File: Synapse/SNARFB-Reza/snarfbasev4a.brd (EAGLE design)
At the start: 80 x 49.5 mm, 67 parts, among them J1 AVR_SPI_PRG_6PTH, X1 USBSMD

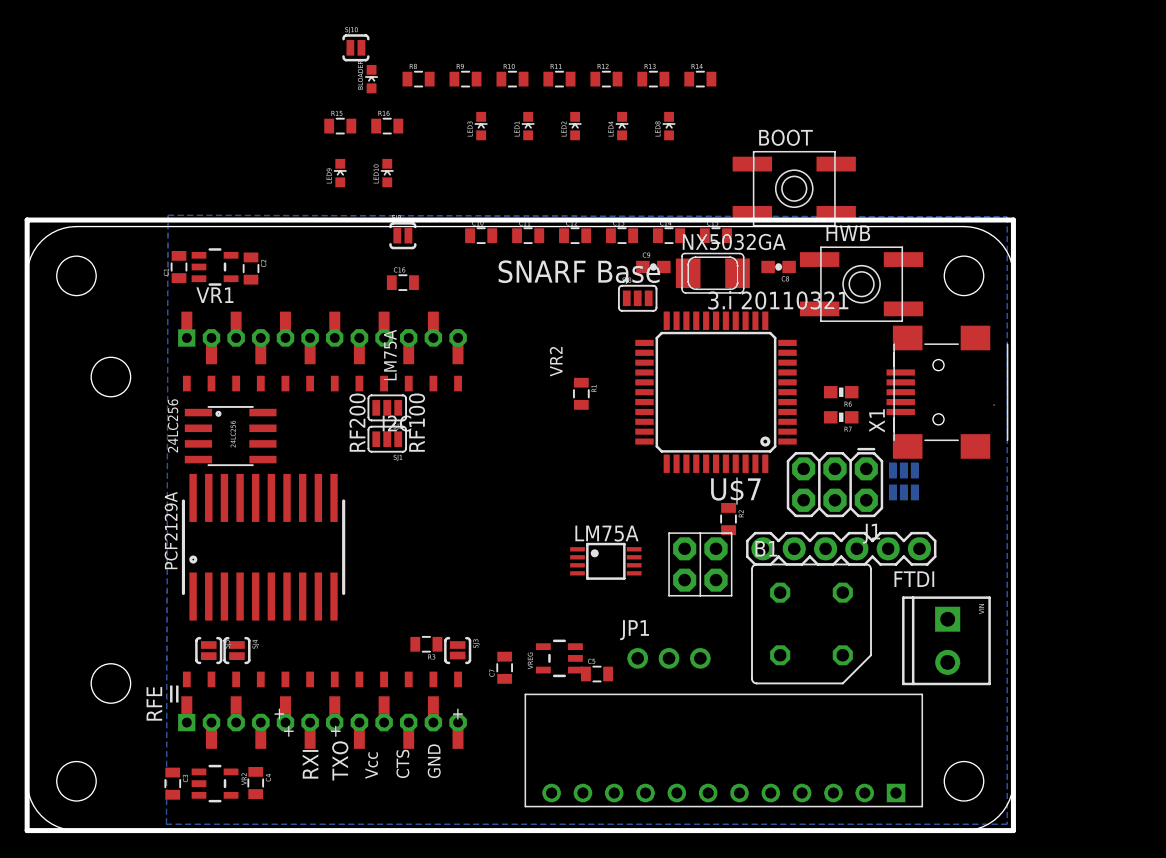
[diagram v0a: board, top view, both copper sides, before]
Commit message: comp sync
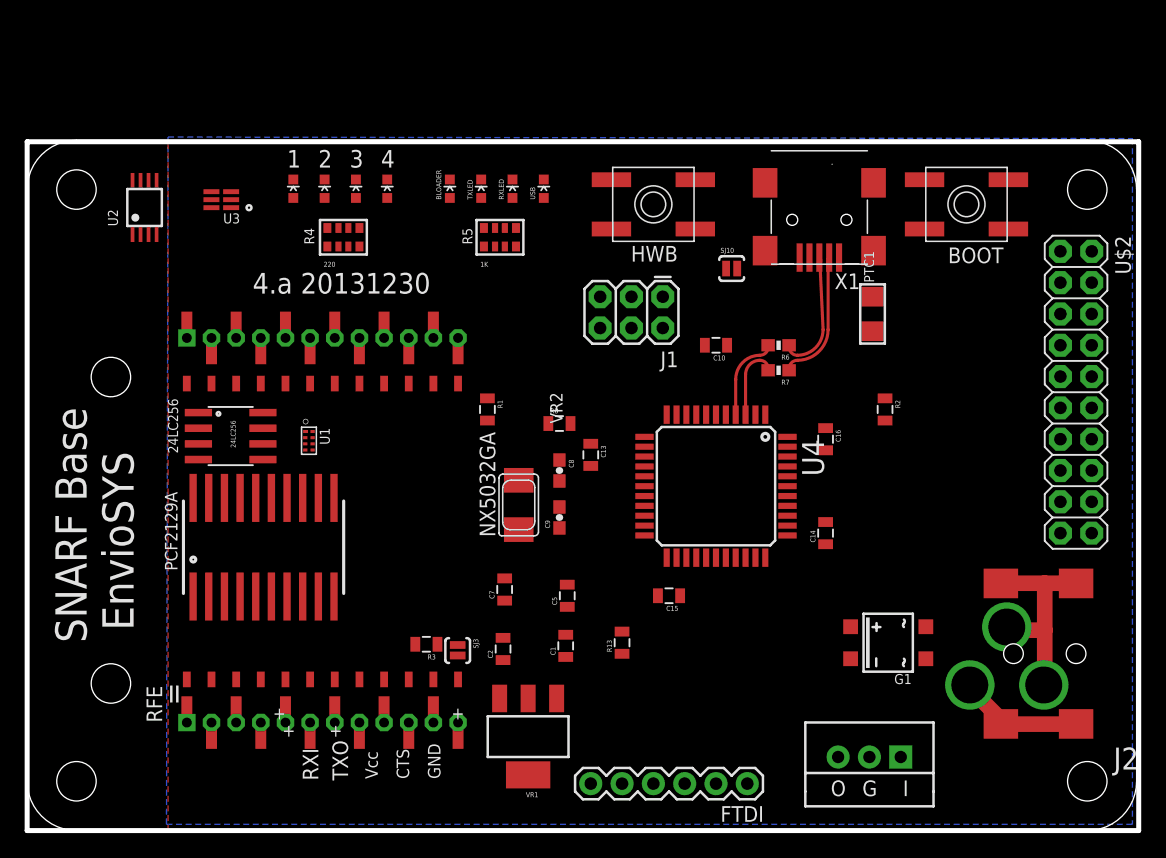
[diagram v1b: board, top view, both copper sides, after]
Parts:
- removed B1: (no value), rectifier:1KAB
- removed C11, C12, C3, C4: 1uF, 0_jc-custom:0805
- removed JP1: (no value), adafruit:1X03-CLEANBIG
- removed LED1: red, 0_jc-custom:LED-0603
- removed LED10: GREEN, 0_jc-custom:LED-0603
- removed LED2: blue, 0_jc-custom:LED-0603
- removed LED3: orange, 0_jc-custom:LED-0603
- removed LED4: green, 0_jc-custom:LED-0603
- removed LED8, LED9: RED, 0_jc-custom:LED-0603
- removed LM75A: LM75AJC-TEST, 0_jc-custom-eagle6:TSSOP8-3MM
- removed PCB1: PCB_DP_RECTANGLE-80X49, dp_pcb:DP8049_V1
- removed R10, R16, R9: 220, SparkFun-Resistors:0805
- removed R11, R12, R14, R15: 1K, SparkFun-Resistors:0805
- removed RXTX: SERIAL_CROSSOVERNORMAL, 0_jc-custom-eagle6:2X02_SXOVER
- removed SJ1, SJ2: (no value), SparkFun:SJ_3
- removed SJ4, SJ5, SJ9: SOLDERJUMPERNO, SparkFun:SJ_2S-NO
- removed SJ6, SJ7: (no value), SparkFun:SJ_3_PASTE1&2
- removed SJ8: (no value), SparkFun:SJ_3_PASTE2&3
- removed U$1: R7XXXDEF, 0_jc-custom-eagle6:1X12_RECOM
- removed U$7: ATMEGA32U4-AU, adafruit:TQFP44
- removed VIN: M023.5MM, SparkFun-Connectors:SCREWTERMINAL-3.5MM-2
- removed VR2, VREG: MCP1802, 0_jc-custom:SOT23-5
- added 1, 2, 3, 4: red, 0_jc-custom:LED-0603
- added G1: (no value), microbuilder:SOIC-4
- added IC1: (no value), 0_jc-custom-eagle6:TO220-MURATA
- added J2: POWER_JACKCOMBO, SparkFun-Connectors:POWER_JACK_COMBO
- added PTC1: (no value), microbuilder:1206
- added R4: 220, microbuilder:RESPACK_4X0603
- added R5: 1K, microbuilder:RESPACK_4X0603
- added RXLED, TXLED: yellow, 0_jc-custom:LED-0603
- added U$2: M10X2, SparkFun-Connectors:2X10
- added U$3: (no value), dp_pcb:DP9056_V1
- added U1: (no value), microbuilder:SOT833-1
- added U2: lm75adp, microbuilder:TSSOP8
- added U3: TSL2561_DFN, microbuilder:TSL2561_FN
- added U4: ATMEGA32U4-AU, adafruit:TQFP44
- added USB: GREEN, 0_jc-custom:LED-0603
- R3: value (none) -> 10k
- R8: value 220 -> 10K
- VR1: value MCP1802 -> MCP1826S; device 0_jc-custom:SOT23-5 -> SparkFun-PowerIC:SOT223
- moved VR1 45.8 mm to (40.6, 7.62), turned to 180 degrees
- moved R13 45.8 mm to (48.3, 15.2), turned to 90 degrees
- moved C1 43.9 mm to (43.7, 15.0)
- moved C2 37.0 mm to (38.6, 14.7), turned to 90 degrees
- moved C16 36.6 mm to (64.8, 31.8), turned to 270 degrees
- moved SJ10 35.4 mm to (57.1, 45.6)
- moved R8 30.2 mm to (43.2, 33.0)
- moved C15 29.5 mm to (52.1, 19.1), turned to 180 degrees
- moved C14 27.3 mm to (64.8, 24.1), turned to 90 degrees
- moved NX5032GA 24.5 mm to (39.9, 26.4), turned to 90 degrees
- moved C8 24.3 mm to (43.2, 29.2), turned to 270 degrees
- moved FTDI 23.6 mm to (58.4, 3.81)
- moved C9 21.7 mm to (43.2, 25.4), turned to 90 degrees
- moved J1 21.6 mm to (51.6, 43.3)
- moved C10 21.0 mm to (55.9, 39.4), turned to 180 degrees
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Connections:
- net UDM renamed UDM_N
- net UDP renamed UDM_P
- removed net 12VUNREG: B1.+, U$1.P$2, U$1.P$3, U$1.P$4
- removed net 24VAC1: B1.AC2, VIN.1
- removed net 24VAC2: B1.AC1, VIN.2
- removed net FTDI_GND: FTDI.6, SJ7.2
- removed net FTDI_VCC: FTDI.4, SJ6.2
- removed net GPIO10: RFE.12, RFE.P12, RFE.P212, SJ3.2
- removed net GPIO17: RFE.19, RFE.P19, RFE.P219, SJ2.3
- removed net GPIO18: RFE.20, RFE.P20, RFE.P220, SJ1.3
- removed net GPIO7: RFE.9, RFE.P209, RFE.P9, RXTX.4
- removed net GPIO8: RFE.10, RFE.P10, RFE.P210, RXTX.1
- removed net GPIO9: FTDI.5, RFE.11, RFE.P11, RFE.P211
- removed net MVOUT: C12.1, R11.2, SJ9.1, VREG.5
- removed net N$13: LED4.A, R16.2
- removed net PB4-GRN-L4: R16.1, U$7.28
- removed net PB5-ORANGE-L3: R10.1, U$7.29
- removed net PB6-BLUE-L2: R9.1, U$7.30
- removed net PB7-RED-L1: R8.1, U$7.12
- removed net PC6-LED8: LED8.A, U$7.31
- removed net PC7-LED9: LED9.A, U$7.32
- removed net PD4: U$7.25
- removed net PD5: U$7.22
- removed net PD6: U$7.26
- removed net PD7: U$7.27
- removed net PE6-LED7-BOOTLOADER: BLOADER.A, U$7.1
- removed net PF0-2: U$7.41
- removed net PF1-3: U$7.40
- removed net PF4-4: U$7.39
- removed net PF5-5: U$7.38
- removed net PF6-6: U$7.37
- removed net PF7-7: U$7.36
- removed net SCL: 24LC256.6, LM75A.2, PCF2129A.P$1, R1.1, SJ1.2, SJ4.1, U$7.18
- removed net SDA: 24LC256.5, LM75A.1, PCF2129A.P$4, R2.1, SJ2.2, SJ5.1, U$7.19
- removed net SD_CS: U$7.8
- removed net UD+: R6.2, U$7.4
- removed net UD-: R7.2, U$7.3
- removed net VCC3A: C4.1, VR2.5
- new net ARXLED: RXLED.C, U4.8
- new net ATXLED: TXLED.C, U4.22
- new net LINT: U3.INT
- new net N$12: 4.A, R4.5
- new net N$3: G1.~1, J2.POWER
- new net PB4-L4-D8: R4.4, U4.28
- new net PB5-L3-D9: R4.3, U4.29
- new net PB6-L2-D10: R4.2, U4.30
- new net PB7-L1-D11: R4.1, U4.12
- new net PC6-D5: U$2.16, U4.31
- new net PC7-D13-LED9BLOAD: BLOADER.C, U4.32
- new net PD4-D4-GPIO10: RFE.12, RFE.P12, RFE.P212, U4.25
- new net PD6-D12-I2COE: U1.6, U4.26
- new net PD7-D6: U$2.18, U4.27
- new net PE6-D7-GPIO9: FTDI.5, RFE.11, RFE.P11, RFE.P211, U4.1
- new net PF0-A5: U$2.4, U4.41
- new net PF1-A4: U$2.6, U4.40
- new net PF4-A3: U$2.8, U4.39
- new net PF5-A2: U$2.10, U4.38
- new net PF6-A1: U$2.12, U4.37
- new net PF7-A0: U$2.14, U4.36
- new net SCL3: 24LC256.6, PCF2129A.P$1, R1.1, RFE.20, RFE.P20, RFE.P220, U1.4, U2.2, U3.CLK
- new net SCL5: U1.1, U4.18
- new net SDA3: 24LC256.5, PCF2129A.P$4, R2.1, RFE.19, RFE.P19, RFE.P219, U1.5, U2.1, U3.DATA
- new net SDA5: U1.8, U4.19
- new net UD_N: R7.2, U4.3
- new net UD_P: R6.2, U4.4
- new net VBUSRAW: PTC1.2, X1.VBUS
- net AREF-7: now also U4.42; no longer U$7.42
- net GND: now also 1.C, 2.C, 3.C, 4.C, FTDI.6, G1.-, IC1.GND, U$2.19, U$2.20, U1.2, U2.4, U2.5, U2.6, U2.7, U3.ADR, U3.VSS, U4.15, U4.23, U4.35, U4.43, U4.5, USB.C, VR1.4; no longer B1.-, C11.2, C12.2, C3.2, C4.2, JP1.2, LED1.C, LED10.C, LED2.C, LED3.C, LED4.C, LM75A.4, LM75A.5, LM75A.6, LM75A.7, R12.2, R14.2, R15.2, SJ6.3, SJ7.1, U$1.P$5, U$1.P$6, U$1.P$7, U$1.P$8, U$7.15, U$7.23, U$7.35, U$7.43, U$7.5, VR2.2, VREG.2, X1.GND
- net GPIO0: now also SJ3.2; no longer SJ5.2
- net GPIO1: now also U2.3; no longer SJ4.2
- net GPIO11: no longer SJ1.1
- net GPIO12: no longer SJ2.1
- net GPIO13: now also U$2.15
- net GPIO14: now also U$2.13
- net GPIO15: now also U$2.9
- net GPIO16: now also U$2.11
- net GPIO2: now also U$2.3
- net GPIO5: now also U$2.5; no longer VR2.3
- net GPIO6: now also U$2.7
- net HWB: now also U4.33; no longer U$7.33
- net MISO: now also U4.11; no longer U$7.11
- net MOSI: now also U4.10; no longer U$7.10
- net N$1: now also 1.A, R4.8; no longer LED2.A, R9.2
- net N$10: now also R5.5, USB.A; no longer BLOADER.C, R12.1
- net N$11: now also X1.GND; no longer LM75A.3
- net N$2: now also 2.A, R4.7; no longer LED3.A, R10.2
- net N$4: now also U4.6; no longer U$7.6
- net N$5: now also BLOADER.A, R5.8; no longer LED9.C, R15.1
- net N$6: now also 3.A, R4.6; no longer LED1.A, R8.2
- net N$7: now also G1.~2, J2.GND, J2.GND@1; no longer FTDI.1
- net N$8: now also R5.7, TXLED.A; no longer LED10.A, R11.1
- net N$9: now also R5.6, RXLED.A; no longer LED8.C, R14.1
- net RESET_L: now also FTDI.1
- net RST: now also R8.1, U4.13; no longer U$7.13
- net RX1: now also U4.21; no longer U$7.21
- net RXI: now also FTDI.3, RFE.9, RFE.P209, RFE.P9; no longer FTDI.2, RXTX.3
- net SCK: now also U4.9; no longer U$7.9
- net TX1: now also U4.20; no longer U$7.20
- net TXO: now also FTDI.2, RFE.10, RFE.P10, RFE.P210; no longer FTDI.3, RXTX.2
- net UVCC: now also U1.7; no longer SJ8.2, U$7.2
- net VBUS: now also PTC1.1, R5.1, R5.2, R5.3, R5.4, U4.7; no longer C11.1, SJ8.1, U$7.7, VREG.1, VREG.3, X1.VBUS
- net VCC12: now also G1.+, IC1.IN, U$2.17; no longer JP1.1, U$1.P$10, U$1.P$11, U$1.P$9
- net VCC3: now also FTDI.4, R8.2, U$2.1, U1.3, U2.8, U3.VDD, U4.14, U4.2, U4.24, U4.34, U4.44, VR1.3; no longer LM75A.8, SJ6.1, SJ7.3, SJ8.3, SJ9.2, U$7.14, U$7.24, U$7.34, U$7.44, VR1.5
- net VCC5: now also IC1.OUT, U$2.2; no longer C3.1, JP1.3, VR1.3, VR2.1
- net XTAL1: now also U4.17; no longer U$7.17
- net XTAL2: now also U4.16; no longer U$7.16
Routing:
- net UDM_N: track 0.00 -> 10.5 mm
- net UDM_P: track 0.00 -> 9.89 mm
- net UD_P: track 0.00 -> 6.68 mm
- net UD_N: track 0.00 -> 5.95 mm
- added copper zone on layer 1, net GND
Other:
- board size 80 x 49.5 mm -> 90.2 x 55.9 mm
- board text added: "4.a 20131230"
- board text added: "SNARF Base EnvioSYS"
- board text removed: "3.i 20110321"
- board text removed: "I2C"
- board text removed: "LM75A"
- board text removed: "RF100"
- board text removed: "RF200"
- board text removed: "SNARF Base"

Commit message: prep for submission
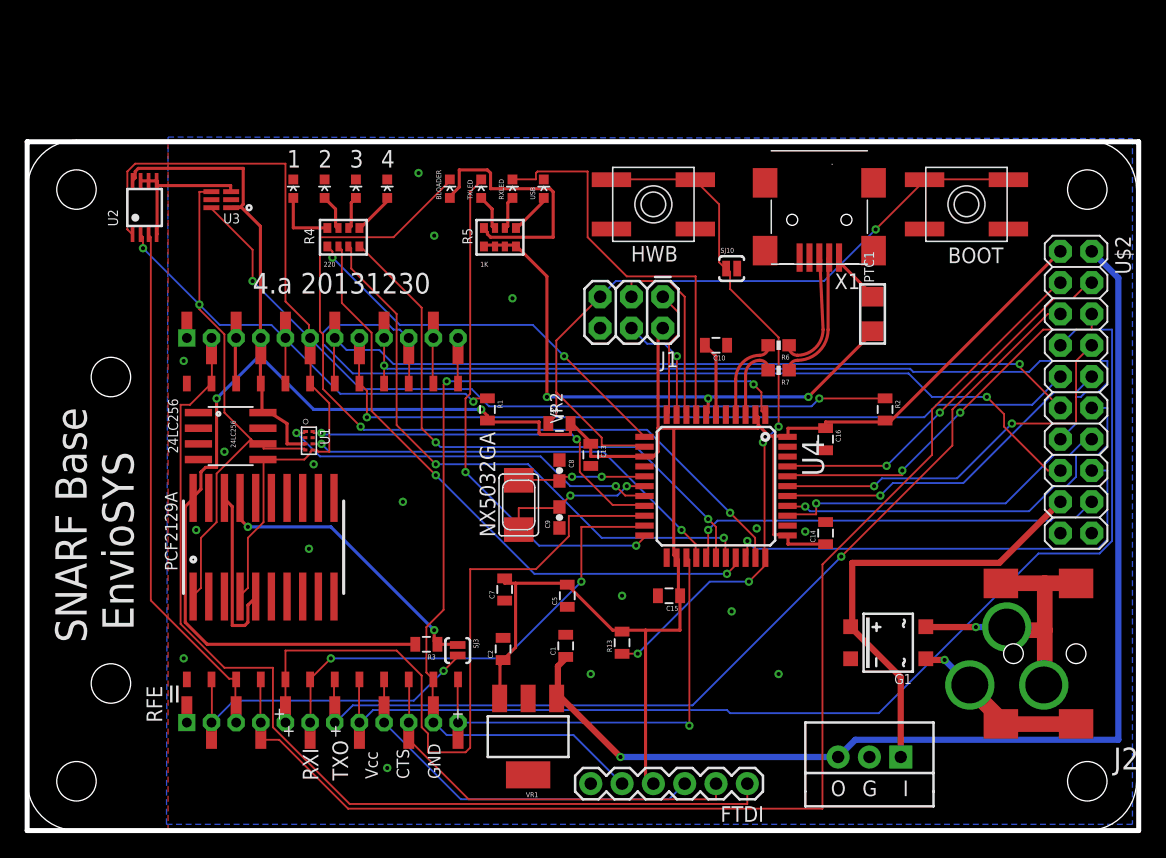
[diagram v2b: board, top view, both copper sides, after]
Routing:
- net VCC3: track 0.00 -> 240.5 mm, vias 0 -> 2
- net SDA3: track 0.00 -> 124.1 mm, vias 0 -> 2
- net GPIO2: track 0.00 -> 103.5 mm
- net GPIO6: track 0.00 -> 94.1 mm
- net VCC5: track 0.00 -> 92.4 mm, vias 0 -> 1
- net SCL3: track 0.00 -> 82.1 mm, vias 0 -> 3
- net RESET_L: track 0.00 -> 81.2 mm
- net GPIO5: track 0.00 -> 77.9 mm, vias 0 -> 1
- net GPIO13: track 0.00 -> 77.0 mm, vias 0 -> 1
- net PE6-D7-GPIO9: track 0.00 -> 74.0 mm, vias 0 -> 2
- net GPIO14: track 0.00 -> 73.0 mm, vias 0 -> 1
- net PC7-D13-LED9BLOAD: track 0.00 -> 66.6 mm, vias 0 -> 2
- net GPIO16: track 0.00 -> 66.5 mm, vias 0 -> 1
- net GPIO15: track 0.00 -> 64.4 mm, vias 0 -> 1
- net TX1: track 0.00 -> 59.1 mm
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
